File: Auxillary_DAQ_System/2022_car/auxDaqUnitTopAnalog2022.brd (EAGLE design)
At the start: 25.4 x 193 mm, 17 parts

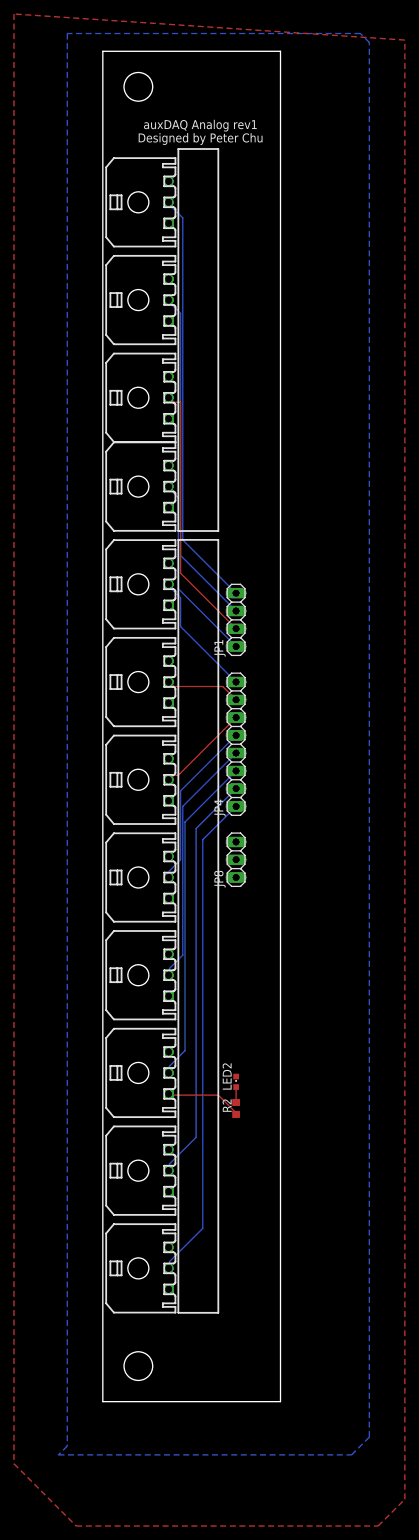
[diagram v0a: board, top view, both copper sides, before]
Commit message: Mostly done with Aux Daq Rework
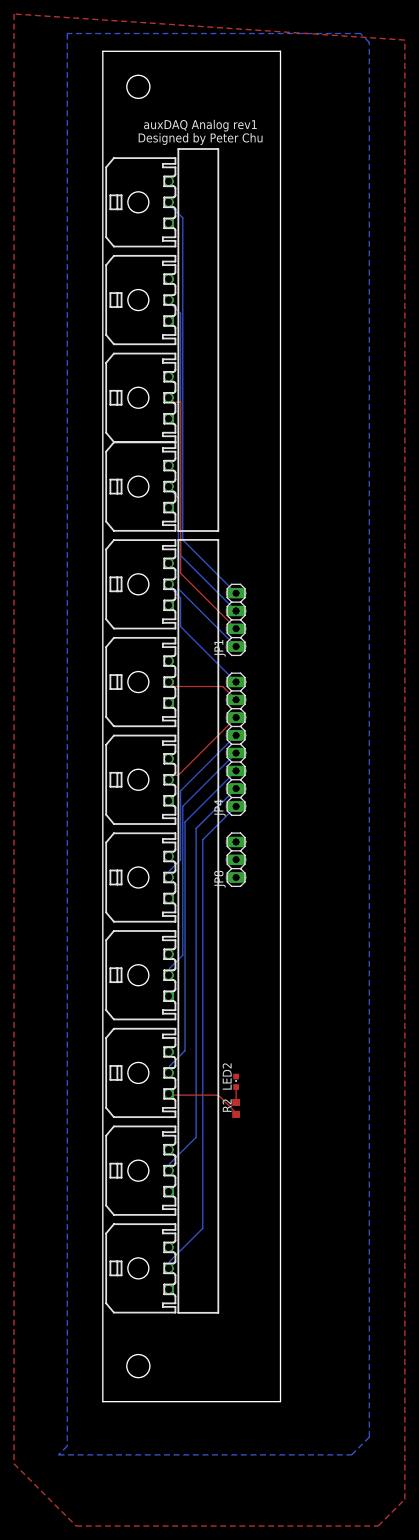
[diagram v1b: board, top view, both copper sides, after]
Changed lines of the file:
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@@
 <wire x1="36.83" y1="193.04" x2="11.43" y2="193.04" width="0" layer="20"/>
 <wire x1="11.43" y1="193.04" x2="11.43" y2="0" width="0" layer="20"/>
-<hole x="16.51" y="187.96" drill="4.1"/>
-<hole x="16.51" y="5.08" drill="4.1"/>
+<hole x="16.51" y="187.96" drill="3.3"/>
+<hole x="16.51" y="5.08" drill="3.3"/>
 <text x="25.4" y="181.61" size="1.27" layer="25" rot="SR0" align="center">auxDAQ Analog rev1
 Designed by Peter Chu</text>
